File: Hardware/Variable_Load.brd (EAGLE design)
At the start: 125.7 x 41.9 mm, 53 parts, among them J3 AMP FCI 10103594-0001LF, Q1 60V/32A/35mΩ, U1 CY8C5868LTI-LP039, U2 3.3V

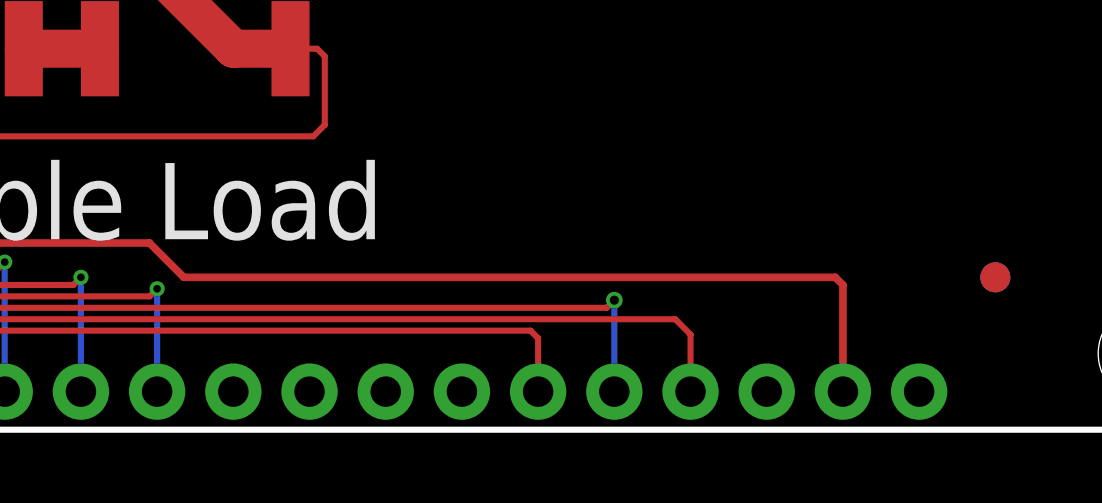
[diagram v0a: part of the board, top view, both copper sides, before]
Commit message: Changes for 2nd proto round
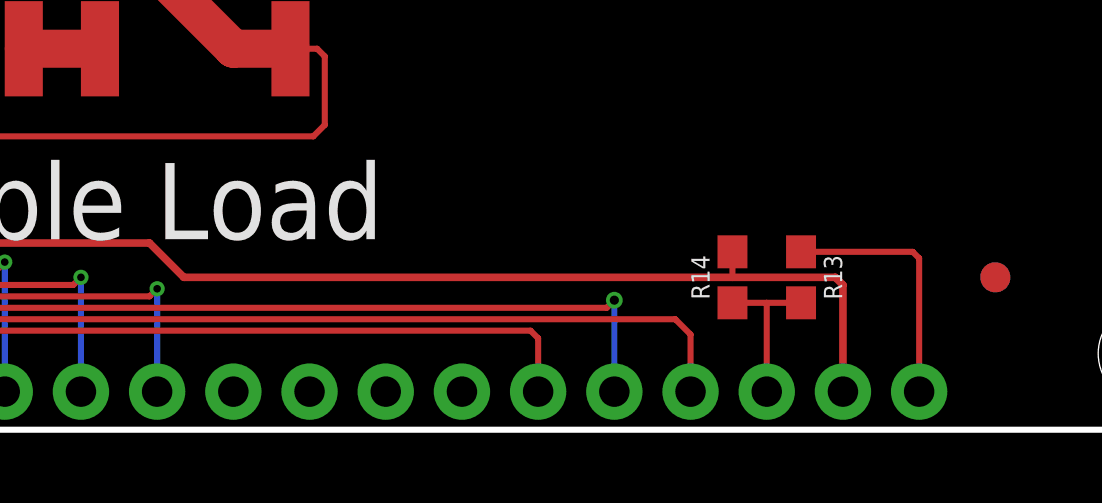
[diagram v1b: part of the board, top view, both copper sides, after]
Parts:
- added R13: 1k, SparkFun-Resistors:0603
- added R14: 4.7k, SparkFun-Resistors:0603
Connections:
- new net CONTRAST: J2.3, R13.2, R14.1
- net 5V: now also R14.2
- net GND: now also R13.1; no longer J2.3
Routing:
- net GND: track 57.2 -> 65.7 mm
- net CONTRAST: track 0.00 -> 5.25 mm
- net 5V: track 185.7 -> 186.5 mm
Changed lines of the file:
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@@
 <layer number="20" name="Dimension" color="15" fill="1" visible="yes" active="yes"/>
 <layer number="21" name="tPlace" color="16" fill="1" visible="yes" active="yes"/>
-<layer number="22" name="bPlace" color="14" fill="1" visible="no" active="yes"/>
+<layer number="22" name="bPlace" color="14" fill="1" visible="yes" active="yes"/>
 <layer number="23" name="tOrigins" color="15" fill="1" visible="yes" active="yes"/>
-<layer number="24" name="bOrigins" color="15" fill="1" visible="no" active="yes"/>
-<layer number="25" name="tNames" color="7" fill="1" visible="yes" active="yes"/>
+<layer number="24" name="bOrigins" color="15" fill="1" visible="yes" active="yes"/>
+<layer number="25" name="tNames" color="7" fill="1" visible="no" active="yes"/>
 <layer number="26" name="bNames" color="7" fill="1" visible="no" active="yes"/>
 <layer number="27" name="tValues" color="7" fill="1" visible="no" active="yes"/>
@@
 <layer number="43" name="vRestrict" color="2" fill="10" visible="no" active="yes"/>
 <layer number="44" name="Drills" color="7" fill="1" visible="no" active="yes"/>
-<layer number="45" name="Holes" color="7" fill="1" visible="no" active="yes"/>
+<layer number="45" name="Holes" color="7" fill="1" visible="yes" active="yes"/>
 <layer number="46" name="Milling" color="3" fill="1" visible="no" active="yes"/>
 <layer number="47" name="Measures" color="7" fill="1" visible="no" active="yes"/>
 <layer number="48" name="Document" color="7" fill="1" visible="no" active="yes"/>
 <layer number="49" name="Reference" color="7" fill="1" visible="no" active="yes"/>
-<layer number="51" name="tDocu" color="6" fill="1" visible="no" active="yes"/>
+<layer number="51" name="tDocu" color="6" fill="1" visible="yes" active="yes"/>
 <layer number="52" name="bDocu" color="7" fill="1" visible="no" active="yes"/>
 <layer number="3" name="Route3" color="4" fill="3" visible="no" active="no"/>
@@
 <attribute name="PROD_ID" value="RES-13766" x="35.56" y="26.67" size="1.778" layer="27" font="vector" ratio="15" rot="R90" display="off"/>
 </element>
+<element name="R13" library="SparkFun-Resistors" package="0603" value="1k" x="111.633" y="5.08" rot="R270">
+<attribute name="PROD_ID" value="RES-07856" x="111.633" y="5.08" size="1.778" layer="27" font="vector" ratio="15" rot="R270" display="off"/>
+</element>
+<element name="R14" library="SparkFun-Resistors" package="0603" value="4.7k" x="109.347" y="5.08" rot="R90">
+<attribute name="PROD_ID" value="RES-07857" x="109.347" y="5.08" size="1.778" layer="27" font="vector" ratio="15" rot="R90" display="off"/>
+</element>
 </elements>
 <signals>
@@
 <contactref element="U1" pad="25"/>
 <contactref element="J2" pad="1"/>
-<contactref element="J2" pad="3"/>
 <contactref element="J3" pad="GND"/>
 <contactref element="U2" pad="2"/>
@@
 <wire x1="17.71858125" y1="37.65808125" x2="17.71858125" y2="36.00658125" width="0.254" layer="1"/>
 <wire x1="17.71858125" y1="36.00658125" x2="17.526" y2="35.814" width="0.254" layer="1"/>
+<contactref element="R13" pad="1"/>
+<wire x1="111.633" y1="5.93" x2="115.355" y2="5.93" width="0.2032" layer="1"/>
+<wire x1="115.355" y1="5.93" x2="115.57" y2="5.715" width="0.2032" layer="1"/>
+<wire x1="115.57" y1="5.715" x2="115.57" y2="1.27" width="0.2032" layer="1"/>
 </signal>
 <signal name="3.3V">
@@
 <wire x1="84.836" y1="6.223" x2="89.916" y2="6.223" width="0.254" layer="1"/>
 <wire x1="89.916" y1="6.223" x2="91.059" y2="5.08" width="0.254" layer="1"/>
-<wire x1="91.059" y1="5.08" x2="112.776" y2="5.08" width="0.254" layer="1"/>
+<wire x1="91.059" y1="5.08" x2="109.347" y2="5.08" width="0.254" layer="1"/>
+<wire x1="109.347" y1="5.08" x2="112.776" y2="5.08" width="0.254" layer="1"/>
 <wire x1="112.776" y1="5.08" x2="113.03" y2="4.826" width="0.254" layer="1"/>
 <wire x1="113.03" y1="4.826" x2="113.03" y2="1.27" width="0.254" layer="1"/>
@@
 <wire x1="22.86" y1="32.128" x2="21.46" y2="32.128" width="0.254" layer="1"/>
 <wire x1="21.46" y1="32.128" x2="21.082" y2="31.75" width="0.254" layer="1"/>
+<contactref element="R14" pad="2"/>
+<wire x1="109.347" y1="5.93" x2="109.347" y2="5.08" width="0.2032" layer="1"/>
 </signal>
 <signal name="N$10">
@@
 <wire x1="35.56" y1="26.09" x2="35.56" y2="23.39" width="0.2032" layer="1"/>
 </signal>
+<signal name="CONTRAST">
+<contactref element="J2" pad="3"/>
+<contactref element="R13" pad="2"/>
+<contactref element="R14" pad="1"/>
+<wire x1="109.347" y1="4.23" x2="110.49" y2="4.23" width="0.2032" layer="1"/>
+<wire x1="110.49" y1="4.23" x2="111.633" y2="4.23" width="0.2032" layer="1"/>
+<wire x1="110.49" y1="1.27" x2="110.49" y2="4.23" width="0.2032" layer="1"/>
+</signal>
 </signals>
